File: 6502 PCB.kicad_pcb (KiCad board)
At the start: 2 copper layers, 111.8 x 83.8 mm, 15 parts, among them J1 power_source, J2 Conn_01x08_Pin, J3 Conn_01x08_Pin, SW1 RESET, U1 W65C02S, U2 28C256, U3 62256, U4 W65C22, U5 74HC00, X1 1MHz

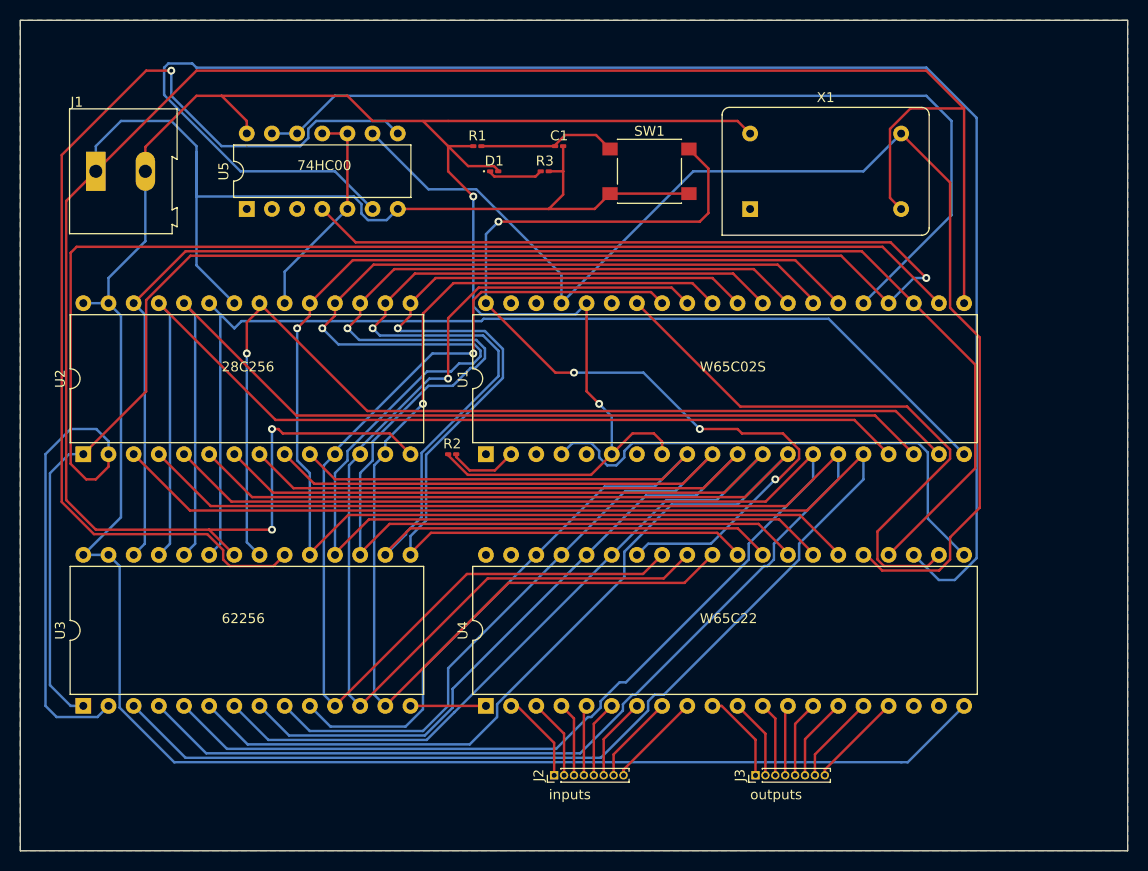
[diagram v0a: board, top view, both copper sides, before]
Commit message: Add files via upload
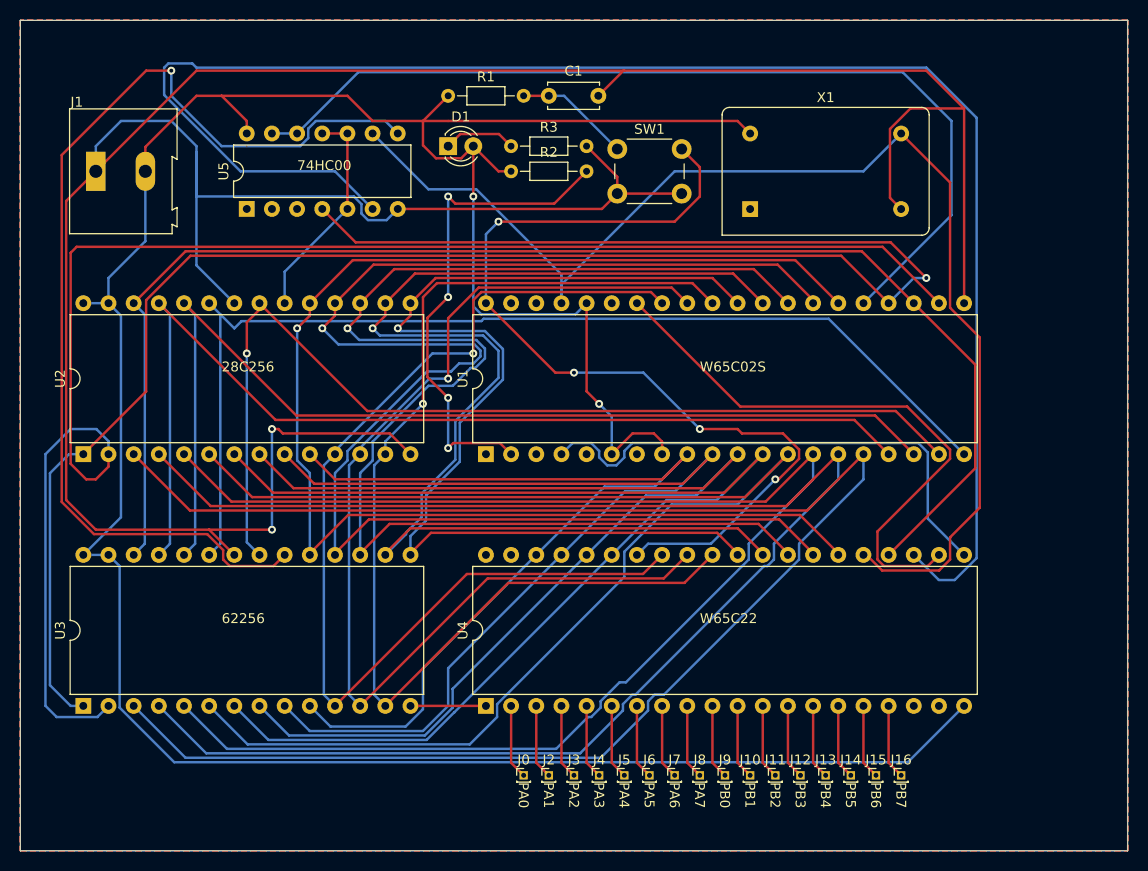
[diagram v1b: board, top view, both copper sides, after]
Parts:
- added J0: Conn_01x01_Pin, Connector_PinHeader_1.00mm:PinHeader_1x01_P1.00mm_Vertical, F.Cu at (63.5, 88.9)
- added J10: Conn_01x01_Pin, Connector_PinHeader_1.00mm:PinHeader_1x01_P1.00mm_Vertical, F.Cu at (86.4, 88.9)
- added J11: Conn_01x01_Pin, Connector_PinHeader_1.00mm:PinHeader_1x01_P1.00mm_Vertical, F.Cu at (88.9, 88.9)
- added J12: Conn_01x01_Pin, Connector_PinHeader_1.00mm:PinHeader_1x01_P1.00mm_Vertical, F.Cu at (91.4, 88.9)
- added J13: Conn_01x01_Pin, Connector_PinHeader_1.00mm:PinHeader_1x01_P1.00mm_Vertical, F.Cu at (94.0, 88.9)
- added J14: Conn_01x01_Pin, Connector_PinHeader_1.00mm:PinHeader_1x01_P1.00mm_Vertical, F.Cu at (96.5, 88.9)
- added J15: Conn_01x01_Pin, Connector_PinHeader_1.00mm:PinHeader_1x01_P1.00mm_Vertical, F.Cu at (99.1, 88.9)
- added J16: Conn_01x01_Pin, Connector_PinHeader_1.00mm:PinHeader_1x01_P1.00mm_Vertical, F.Cu at (101.6, 88.9)
- added J4: Conn_01x01_Pin, Connector_PinHeader_1.00mm:PinHeader_1x01_P1.00mm_Vertical, F.Cu at (71.1, 88.9)
- added J5: Conn_01x01_Pin, Connector_PinHeader_1.00mm:PinHeader_1x01_P1.00mm_Vertical, F.Cu at (73.7, 88.9)
- added J6: Conn_01x01_Pin, Connector_PinHeader_1.00mm:PinHeader_1x01_P1.00mm_Vertical, F.Cu at (76.2, 88.9)
- added J7: Conn_01x01_Pin, Connector_PinHeader_1.00mm:PinHeader_1x01_P1.00mm_Vertical, F.Cu at (78.7, 88.9)
- added J8: Conn_01x01_Pin, Connector_PinHeader_1.00mm:PinHeader_1x01_P1.00mm_Vertical, F.Cu at (81.3, 88.9)
- added J9: Conn_01x01_Pin, Connector_PinHeader_1.00mm:PinHeader_1x01_P1.00mm_Vertical, F.Cu at (83.8, 88.9)
- C1: footprint Capacitor_SMD:C_0201_0603Metric_Pad0.64x0.40mm_HandSolder -> Capacitor_THT:C_Disc_D5.0mm_W2.5mm_P5.00mm
- D1: footprint LED_SMD:LED_0201_0603Metric_Pad0.64x0.40mm_HandSolder -> LED_THT:LED_D3.0mm
- J2, J3: value Conn_01x08_Pin -> Conn_01x01_Pin; footprint Connector_PinHeader_1.00mm:PinHeader_1x08_P1.00mm_Vertical -> Connector_PinHeader_1.00mm:PinHeader_1x01_P1.00mm_Vertical
- R1, R2, R3: footprint Resistor_SMD:R_0201_0603Metric_Pad0.64x0.40mm_HandSolder -> Resistor_THT:R_Axial_DIN0204_L3.6mm_D1.6mm_P7.62mm_Horizontal
- SW1: footprint Button_Switch_SMD:SW_SPST_PTS645 -> Button_Switch_THT:SW_PUSH_6mm
- moved R2 29.2 mm to (62.2, 27.9)
- moved J3 18.3 mm to (68.6, 88.9), turned to 0 degrees
- moved R1 5.87 mm to (55.9, 20.3)
- moved D1 5.30 mm to (55.9, 25.4)
- moved C1 5.19 mm to (66.0, 20.3)
- moved R3 4.25 mm to (62.2, 25.4)
- moved SW1 3.95 mm to (73.0, 25.7)
- moved J2 0.54 mm to (66.0, 88.9), turned to 0 degrees
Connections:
- U4 pad 10: Net-(J3-Pin_1) -> Net-(J9-Pin_1)
- U4 pad 11: Net-(J3-Pin_2) -> Net-(J10-Pin_1)
- U4 pad 12: Net-(J3-Pin_3) -> Net-(J11-Pin_1)
- U4 pad 13: Net-(J3-Pin_4) -> Net-(J12-Pin_1)
- U4 pad 14: Net-(J3-Pin_5) -> Net-(J13-Pin_1)
- U4 pad 15: Net-(J3-Pin_6) -> Net-(J14-Pin_1)
- U4 pad 16: Net-(J3-Pin_7) -> Net-(J15-Pin_1)
- U4 pad 17: Net-(J3-Pin_8) -> Net-(J16-Pin_1)
- U4 pad 2: Net-(J2-Pin_1) -> Net-(J0-Pin_1)
- U4 pad 3: Net-(J2-Pin_2) -> Net-(J2-Pin_1)
- U4 pad 4: Net-(J2-Pin_3) -> Net-(J3-Pin_1)
- U4 pad 5: Net-(J2-Pin_4) -> Net-(J4-Pin_1)
- U4 pad 6: Net-(J2-Pin_5) -> Net-(J5-Pin_1)
- U4 pad 7: Net-(J2-Pin_6) -> Net-(J6-Pin_1)
- U4 pad 8: Net-(J2-Pin_7) -> Net-(J7-Pin_1)
- U4 pad 9: Net-(J2-Pin_8) -> Net-(J8-Pin_1)
- U5 pad 14: /VDD -> (no net)
- U5 pad 7: /GND -> (no net)
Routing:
- net Net-(U1-RDY): track 7.06 -> 49.8 mm, vias 0 -> 4
- net /VDD: track 309.2 -> 294.5 mm
- net Net-(J2-Pin_8): track 9.67 -> 0.00 mm
- net Net-(J3-Pin_8): track 9.67 -> 0.00 mm
- net Net-(J3-Pin_7): track 9.03 -> 0.00 mm
- net Net-(J2-Pin_7): track 9.03 -> 0.00 mm
- net Net-(J2-Pin_6): track 8.39 -> 0.00 mm
- net Net-(J3-Pin_6): track 8.39 -> 0.00 mm
- net Net-(J2-Pin_5): track 8.17 -> 0.00 mm
- net Net-(J3-Pin_2): track 8.17 -> 0.00 mm
- net Net-(J2-Pin_2): track 8.17 -> 0.00 mm
- net Net-(J5-Pin_1): track 0.00 -> 7.94 mm
- net Net-(J3-Pin_5): track 7.76 -> 0.00 mm
- net Net-(J8-Pin_1): track 0.00 -> 7.53 mm
- net Net-(J7-Pin_1): track 0.00 -> 7.53 mm
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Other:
- board text added: "PA0"
- board text added: "PA1"
- board text added: "PA2"
- board text added: "PA3"
- board text added: "PA4"
- board text added: "PA5"
- board text added: "PA6"
- board text added: "PA7"
- board text added: "PB0"
- board text added: "PB1"
- board text added: "PB2"
- board text added: "PB3"
- board text added: "PB4"
- board text added: "PB5"
- board text added: "PB6"
- board text added: "PB7"
- board text removed: "inputs"
- board text removed: "outputs"
